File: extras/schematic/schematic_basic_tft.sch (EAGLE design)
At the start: 18 parts, among them U1 SI4735-D60-GU

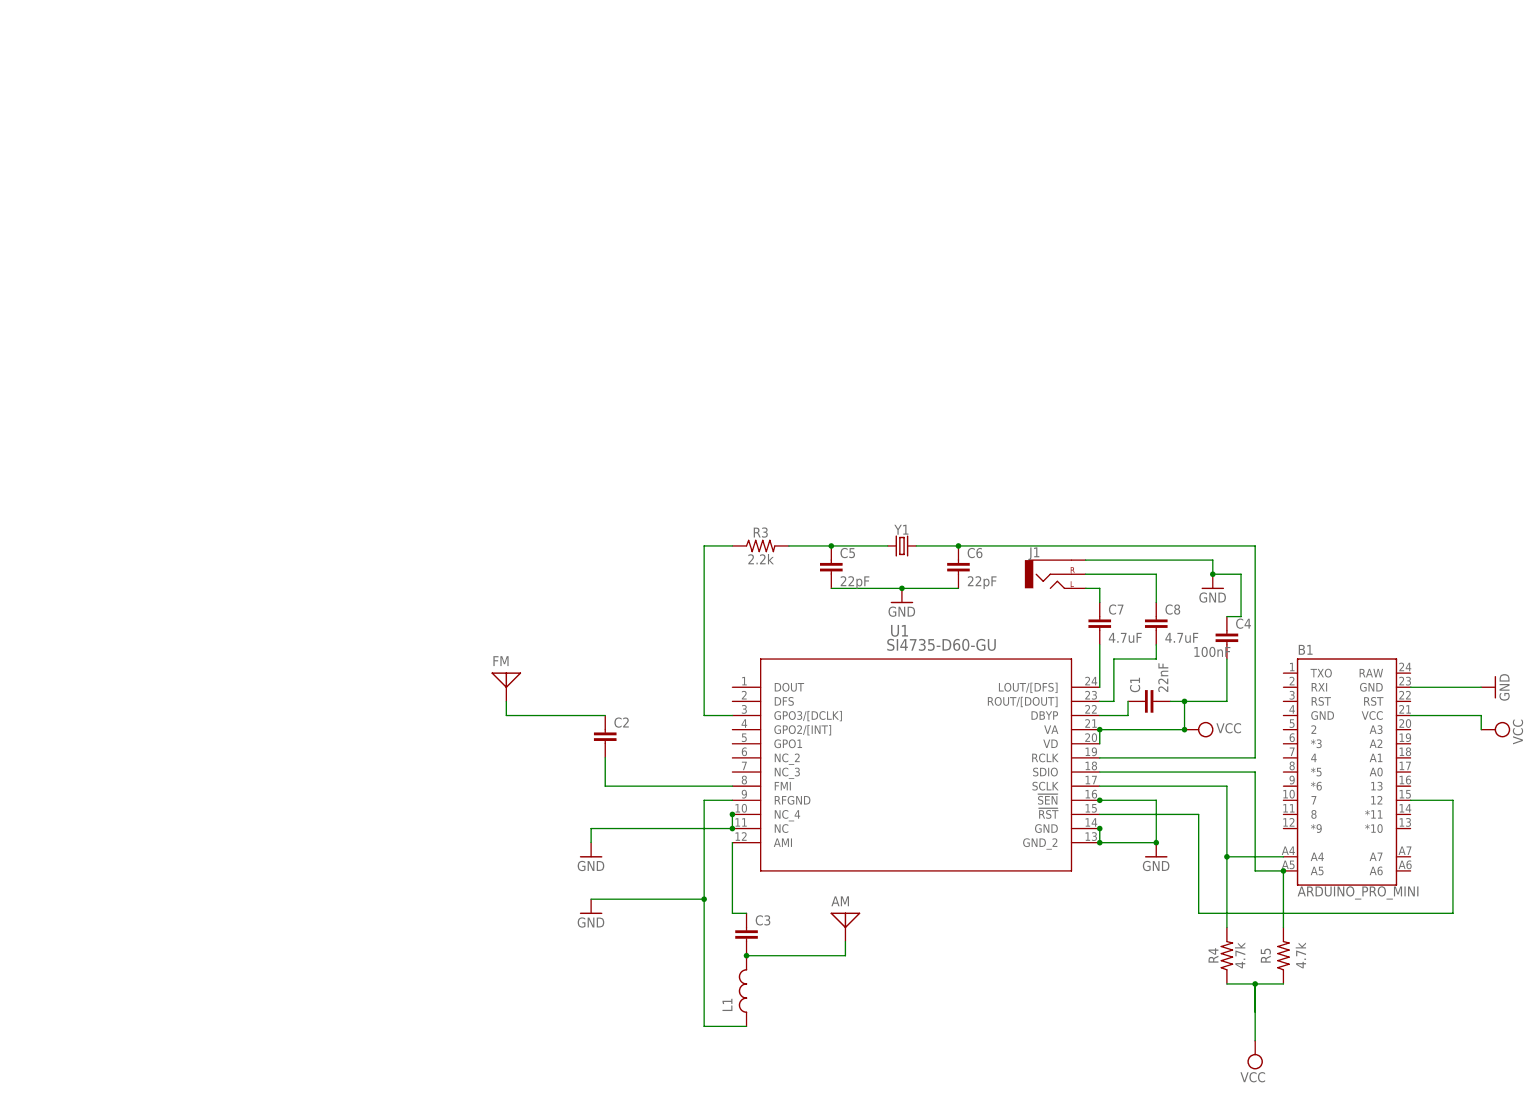
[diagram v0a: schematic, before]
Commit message: SI47XX Arduino Library
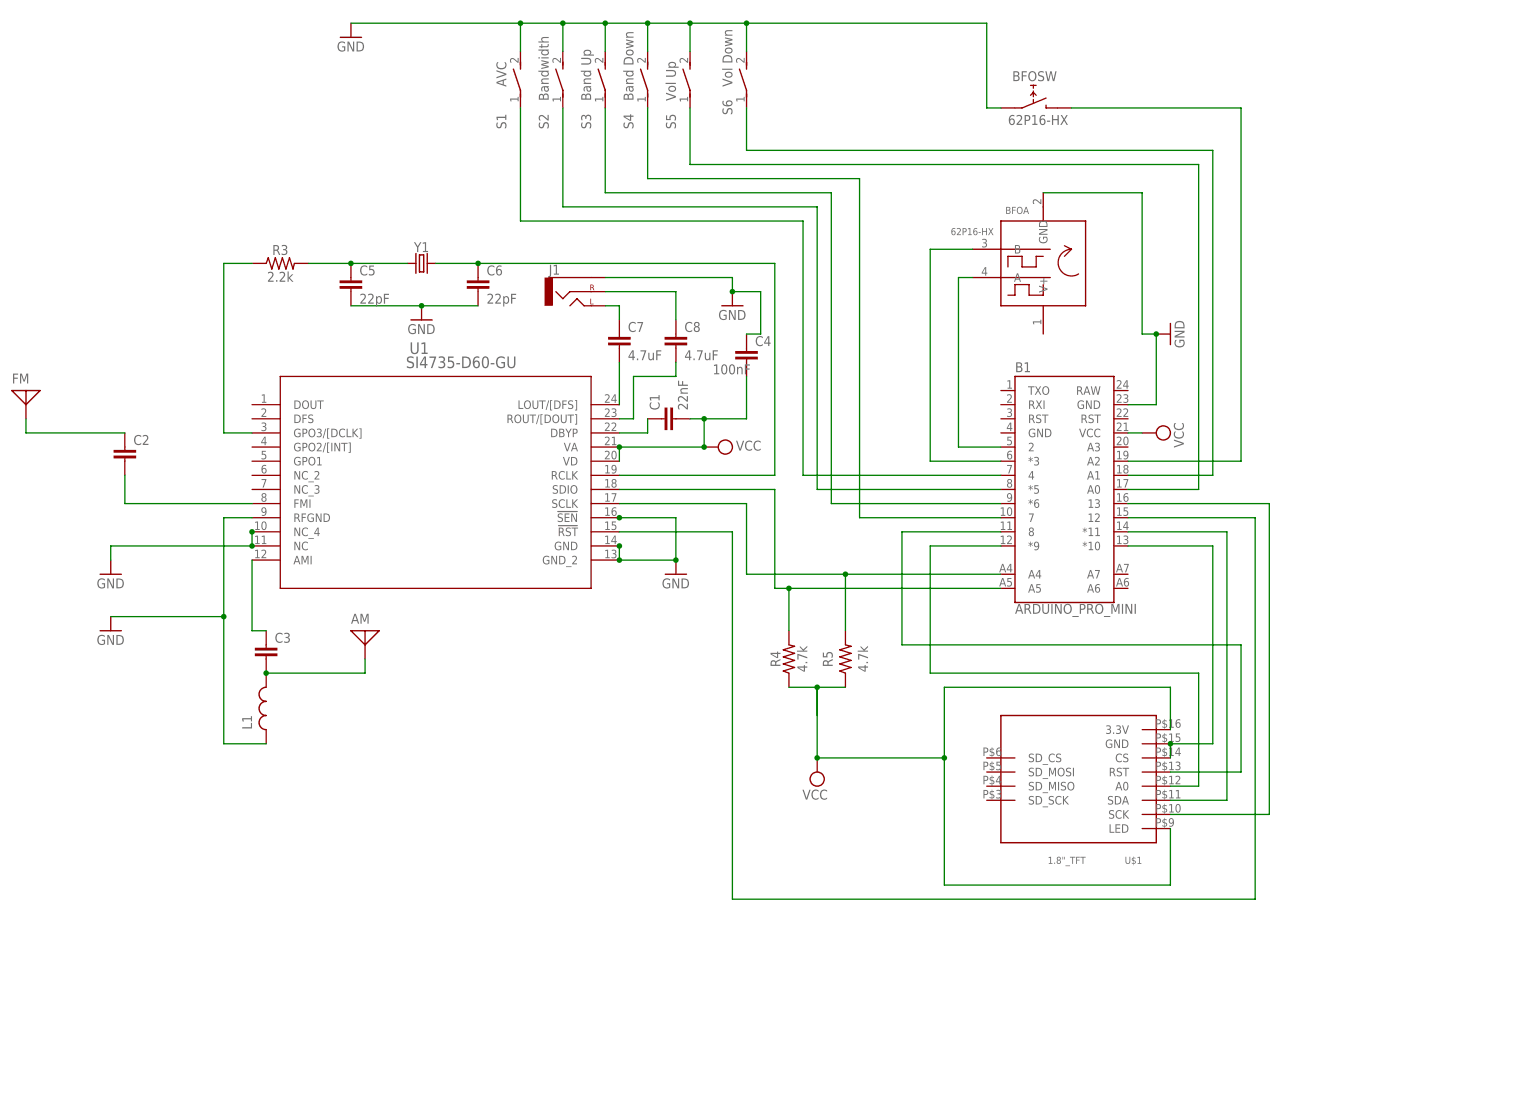
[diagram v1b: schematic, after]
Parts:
- added BFO: 62P16-HX, rotary-encoder:62P16-HX
- added S1: AVC, switch-dil:DS01E
- added S2: Bandwidth, switch-dil:DS01E
- added S3: Band Up, switch-dil:DS01E
- added S4: Band Down, switch-dil:DS01E
- added S5: Vol Up, switch-dil:DS01E
- added S6: Vol Down, switch-dil:DS01E
- added U$1: 1.8"_TFT, tft_1_8_1_44_oled_0_96:1.8"_TFT
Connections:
- new net N$15: B1.2, BFOA.A
- new net N$16: B1.*3, BFOA.B
- new net N$17: B1.4, S1.1
- new net N$18: B1.*5, S2.1
- new net N$19: B1.*6, S3.1
- new net N$20: B1.7, S4.1
- new net N$21: B1.A0, S5.1
- new net N$22: B1.A1, S6.1
- new net N$23: B1.*10, U$1.CS, U$1.GND
- new net N$24: B1.13, U$1.SCK
- new net N$25: B1.8, U$1.RST
- new net N$26: B1.*11, U$1.SDA
- new net N$27: B1.*9, U$1.A0
- new net N$28: B1.A2, BFOSW.E
- net GND: now also BFOA.GND, BFOSW.D, S1.2, S2.2, S3.2, S4.2, S5.2, S6.2
- net N$2: now also R5.2; no longer R4.2
- net SDA: now also R4.2; no longer R5.2
- net VCC: now also U$1.3.3V, U$1.LED
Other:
- moved on the sheet: AM, B1, C1, C2, C3, C4, C5, C6, C7, C8, FM, J1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
